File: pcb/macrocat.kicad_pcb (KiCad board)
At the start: 2 copper layers, 78.7 x 97.3 mm, 52 parts, among them J1 USB-C USB 2.0 MC-372, SW1 SW_Push, SW2 RotaryEncoder_Switch, U1 ATmega32U4-A, Y1 Crystal_GND24_Small

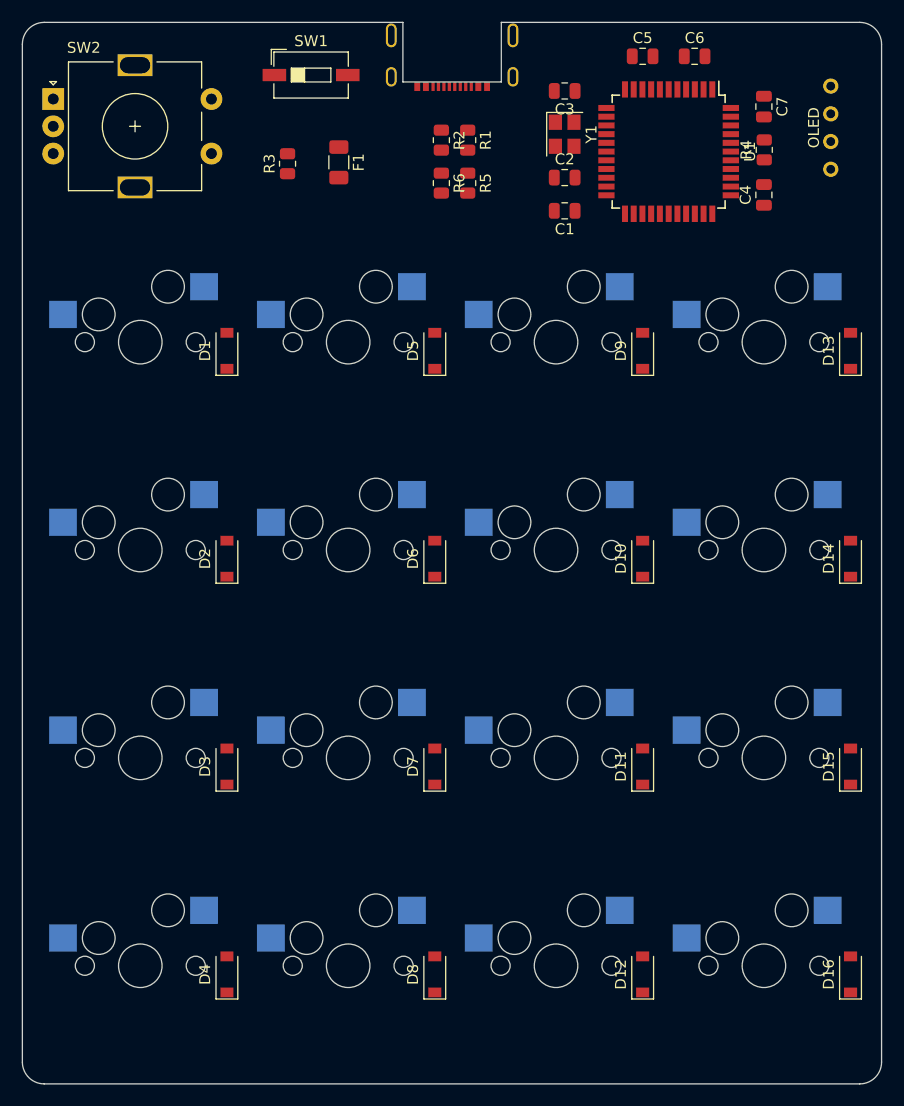
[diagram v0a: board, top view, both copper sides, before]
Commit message: routed by freerouter
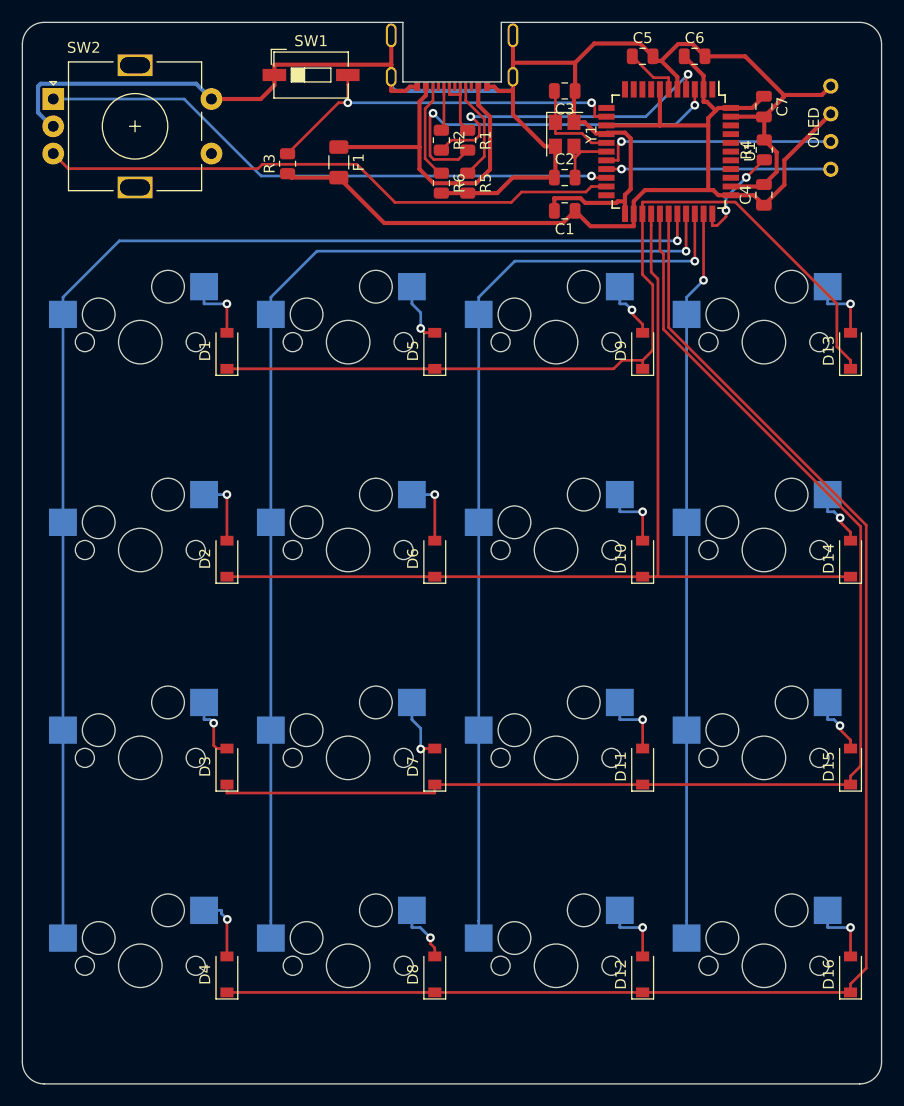
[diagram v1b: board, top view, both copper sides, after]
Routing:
- net GND: track 0.00 -> 168.8 mm
- net ROW4: track 0.00 -> 136.6 mm
- net COL1: track 0.00 -> 119.6 mm, vias 0 -> 1
- net ROW3: track 0.00 -> 119.0 mm
- net COL2: track 0.00 -> 102.0 mm, vias 0 -> 1
- net +5V: track 0.00 -> 92.3 mm
- net ROW2: track 0.00 -> 90.7 mm
- net COL3: track 0.00 -> 84.2 mm, vias 0 -> 1
- net ROW1: track 0.00 -> 82.6 mm
- net COL4: track 0.00 -> 67.0 mm, vias 0 -> 1
- net KNOB1: track 0.00 -> 53.7 mm, vias 0 -> 1
- net KNOB2: track 0.00 -> 53.5 mm
- net Net-(R3-Pad2): track 0.00 -> 34.8 mm, vias 0 -> 2
- net Net-(R1-Pad2): track 0.00 -> 34.6 mm, vias 0 -> 2
- net VCC: track 0.00 -> 30.8 mm
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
